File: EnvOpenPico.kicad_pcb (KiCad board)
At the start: 2 copper layers, 21.1 x 51.3 mm, 38 parts, among them J2 Conn_01x02, J3 Conn_02x18_Odd_Even, J4 Conn_02x18_Odd_Even, J5 Conn_01x03_Male, U1 SPX3819M5-L-3-3, U2 W25Q256JVEIQ_TR, U3 RP2040, X1 XO32

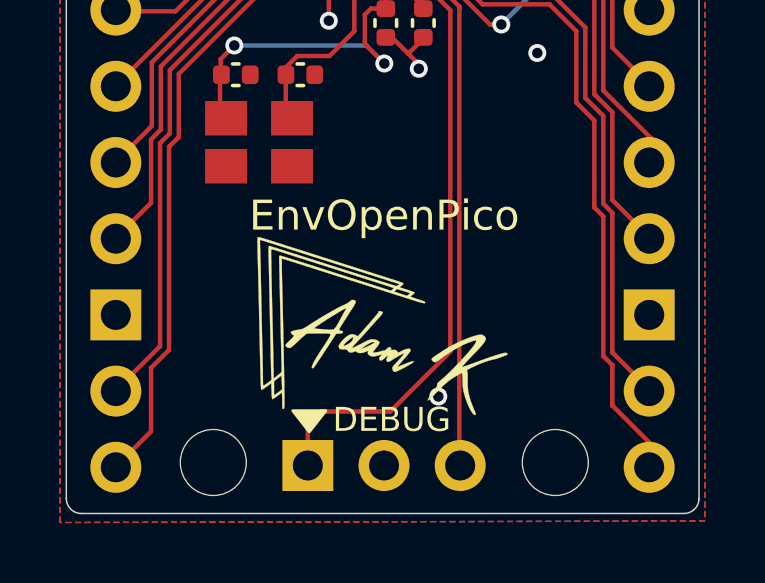
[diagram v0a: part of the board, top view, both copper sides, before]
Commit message: Updated Gerber Files
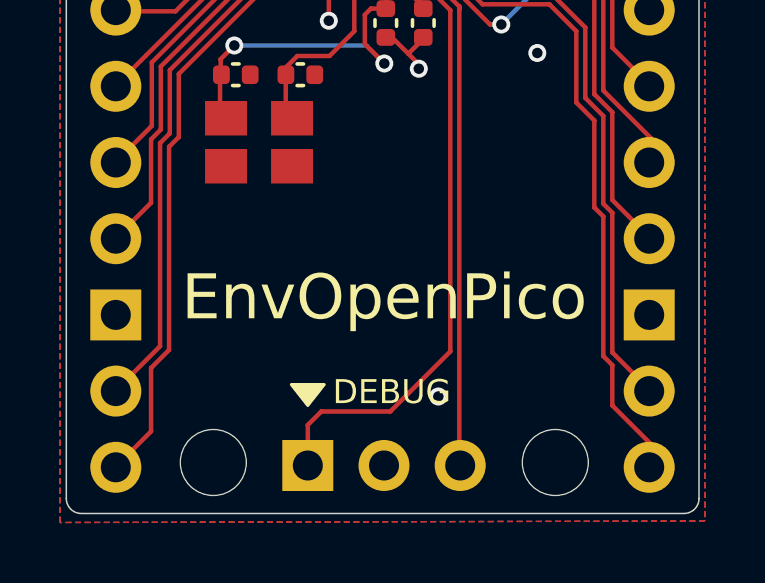
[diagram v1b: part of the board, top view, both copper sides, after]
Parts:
- removed G***: LOGO, EnvExtras:logo
